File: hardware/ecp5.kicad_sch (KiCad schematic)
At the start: 6 parts, among them U3 ECP5U_12_CABGA256

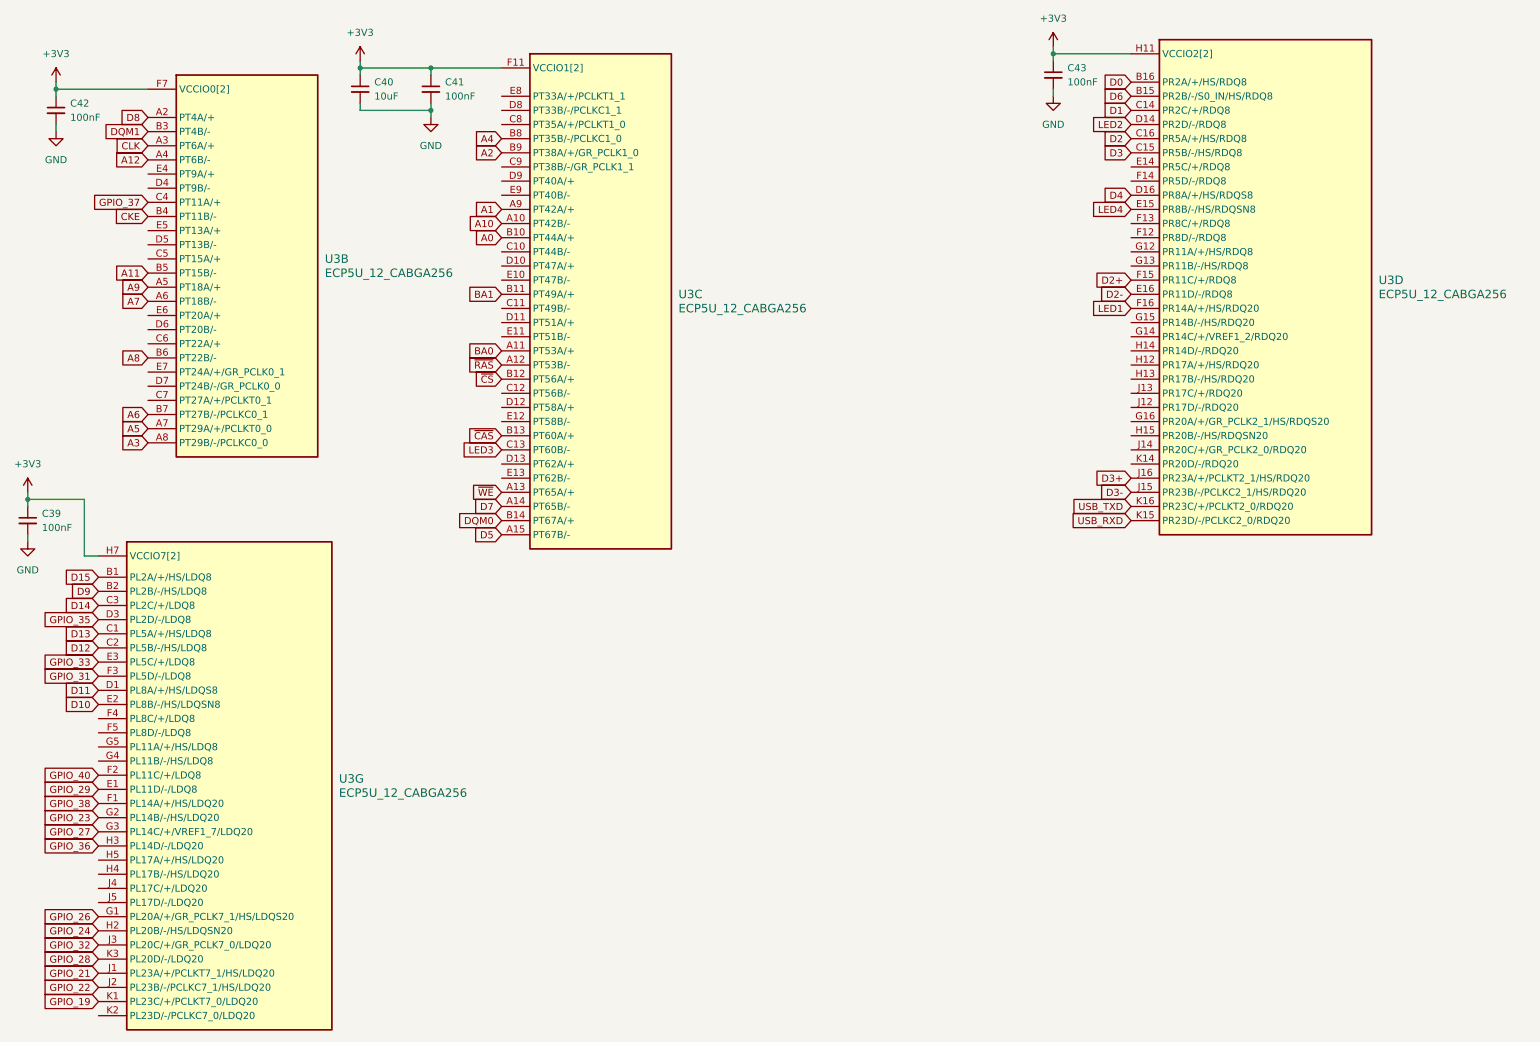
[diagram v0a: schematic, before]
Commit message: Pre-prod fixes
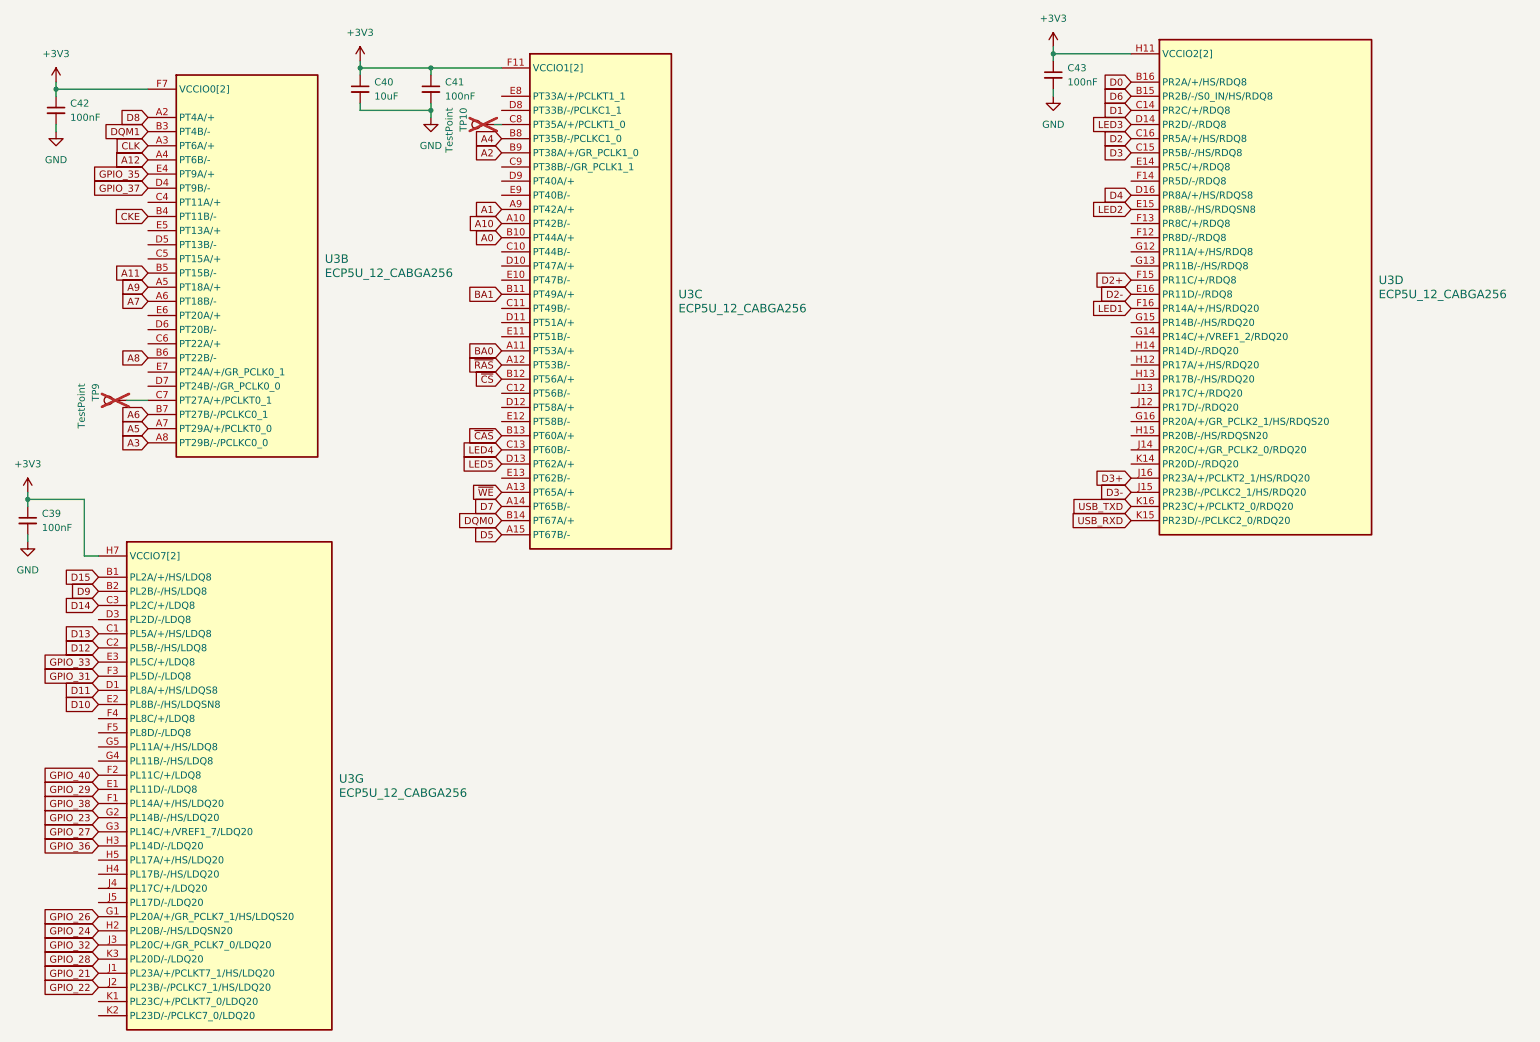
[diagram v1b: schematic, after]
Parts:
- added TP10, TP9: TestPoint, TestPoint:TestPoint_Pad_D2.0mm, symbol Connector:TestPoint
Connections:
- net GPIO_35: now also U3.E4 (PT9A/+); no longer U3.D3 (PL2D/-/LDQ8)
- net GPIO_37: now also U3.D4 (PT9B/-); no longer U3.C4 (PT11A/+)
- net LED2: now also U3.E15 (PR8B/-/HS/RDQSN8); no longer U3.D14 (PR2D/-/RDQ8)
- net LED3: now also U3.D14 (PR2D/-/RDQ8); no longer U3.C13 (PT60B/-)
- net LED4: now also U3.C13 (PT60B/-); no longer U3.E15 (PR8B/-/HS/RDQSN8)
- net at U3.C7 (PT27A/+/PCLKT0_1): now also TP9.1
- net at U3.C8 (PT35A/+/PCLKT1_0): now also TP10.1
- net LED5: now reaches U3.D13 (PT62A/+)
- net GPIO_19: no longer names the net of U3.K1 (PL23C/+/PCLKT7_0/LDQ20)
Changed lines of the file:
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@@
 	(wire
 		(pts
+			(xy 100.33 31.75) (xy 101.6 31.75)
+		)
+		(stroke
+			(width 0)
+			(type default)
+		)
+	)
+	(wire
+		(pts
 			(xy 21.59 31.75) (xy 21.59 33.02)
 		)
@@
 	(wire
 		(pts
+			(xy 34.29 81.28) (xy 38.1 81.28)
+		)
+		(stroke
+			(width 0)
+			(type default)
+		)
+	)
+	(wire
+		(pts
 			(xy 16.51 99.06) (xy 16.51 100.33)
 		)
@@
 		)
 	)
+	(global_label "GPIO_37"
+		(shape input)
+		(at 38.1 43.18 180)
+		(fields_autoplaced yes)
+		(effects
+			(font
+				(size 1.27 1.27)
+			)
+			(justify right)
+		)
+		(property "Intersheetrefs" "${INTERSHEET_REFS}"
+			(at 27.2529 43.18 0)
+			(effects
+				(font
+					(size 1.27 1.27)
+				)
+				(justify right)
+				(hide yes)
+			)
+		)
+	)
 	(global_label "GPIO_23"
 		(shape input)
@@
 		)
 	)
-	(global_label "GPIO_35"
-		(shape input)
-		(at 29.21 120.65 180)
-		(fields_autoplaced yes)
-		(effects
-			(font
-				(size 1.27 1.27)
-			)
-			(justify right)
-		)
-		(property "Intersheetrefs" "${INTERSHEET_REFS}"
-			(at 18.3629 120.65 0)
-			(effects
-				(font
-					(size 1.27 1.27)
-				)
-				(justify right)
-				(hide yes)
-			)
-		)
-	)
 	(global_label "D8"
 		(shape input)
@@
 		)
 	)
-	(global_label "GPIO_24"
+	(global_label "GPIO_35"
 		(shape input)
-		(at 29.21 176.53 180)
+		(at 38.1 40.64 180)
 		(fields_autoplaced yes)
 		(effects
@@
 		)
 		(property "Intersheetrefs" "${INTERSHEET_REFS}"
-			(at 18.3629 176.53 0)
+			(at 27.2529 40.64 0)
 			(effects
 				(font
@@
 		)
 	)
-	(global_label "D3"
+	(global_label "GPIO_24"
 		(shape input)
-		(at 214.63 36.83 180)
+		(at 29.21 176.53 180)
 		(fields_autoplaced yes)
 		(effects
@@
 		)
 		(property "Intersheetrefs" "${INTERSHEET_REFS}"
-			(at 209.1653 36.83 0)
+			(at 18.3629 176.53 0)
 			(effects
 				(font
@@
 		)
 	)
-	(global_label "GPIO_37"
+	(global_label "D3"
 		(shape input)
-		(at 38.1 45.72 180)
+		(at 214.63 36.83 180)
 		(fields_autoplaced yes)
 		(effects
@@
 		)
 		(property "Intersheetrefs" "${INTERSHEET_REFS}"
-			(at 27.2529 45.72 0)
+			(at 209.1653 36.83 0)
 			(effects
 				(font
@@
 		)
 	)
-	(global_label "LED2"
+	(global_label "LED3"
 		(shape input)
 		(at 214.63 31.75 180)
@@
 		)
 	)
-	(global_label "LED4"
+	(global_label "LED2"
 		(shape input)
 		(at 214.63 46.99 180)
@@
 		)
 	)
-	(global_label "GPIO_19"
+	(global_label "A0"
 		(shape input)
-		(at 29.21 189.23 180)
+		(at 101.6 52.07 180)
 		(fields_autoplaced yes)
 		(effects
@@
 		)
 		(property "Intersheetrefs" "${INTERSHEET_REFS}"
-			(at 18.3629 189.23 0)
+			(at 96.3167 52.07 0)
 			(effects
 				(font
@@
 		)
 	)
-	(global_label "A0"
+	(global_label "~{CS}"
 		(shape input)
-		(at 101.6 52.07 180)
+		(at 101.6 77.47 180)
 		(fields_autoplaced yes)
 		(effects
@@
 		)
 		(property "Intersheetrefs" "${INTERSHEET_REFS}"
-			(at 96.3167 52.07 0)
+			(at 96.1353 77.47 0)
 			(effects
 				(font
@@
 		)
 	)
-	(global_label "~{CS}"
+	(global_label "LED5"
 		(shape input)
-		(at 101.6 77.47 180)
+		(at 101.6 92.71 180)
 		(fields_autoplaced yes)
 		(effects
@@
 		)
 		(property "Intersheetrefs" "${INTERSHEET_REFS}"
-			(at 96.1353 77.47 0)
+			(at 93.9582 92.71 0)
 			(effects
 				(font
@@
 		)
 	)
-	(global_label "LED3"
+	(global_label "LED4"
 		(shape input)
 		(at 101.6 90.17 180)
@@
 	)
 	(symbol
+		(lib_id "Connector:TestPoint")
+		(at 34.29 81.28 90)
+		(unit 1)
+		(exclude_from_sim no)
+		(in_bom yes)
+		(on_board yes)
+		(dnp yes)
+		(property "Reference" "TP9"
+			(at 28.702 78.232 0)
+			(effects
+				(font
+					(size 1.27 1.27)
+				)
+				(justify right)
+			)
+		)
+		(property "Value" "TestPoint"
+			(at 26.162 78.232 0)
+			(effects
+				(font
+					(size 1.27 1.27)
+				)
+				(justify right)
+			)
+		)
+		(property "Footprint" "TestPoint:TestPoint_Pad_D2.0mm"
+			(at 34.29 76.2 0)
+			(effects
+				(font
+					(size 1.27 1.27)
+				)
+				(hide yes)
+			)
+		)
+		(property "Datasheet" "~"
+			(at 34.29 76.2 0)
+			(effects
+				(font
+					(size 1.27 1.27)
+				)
+				(hide yes)
+			)
+		)
+		(property "Description" "test point"
+			(at 34.29 81.28 0)
+			(effects
+				(font
+					(size 1.27 1.27)
+				)
+				(hide yes)
+			)
+		)
+		(pin "1"
+		)
+		(instances
+			(project "icepi-zero"
+				(path "/f88da08e-cf42-4d03-a08f-3f602fe6658d/17c9c9b3-f379-4e1f-a876-d3fcf0529a4d"
+					(reference "TP9")
+					(unit 1)
+				)
+			)
+		)
+	)
+	(symbol
 		(lib_id "josh:ECP5U_12_CABGA256")
 		(at 236.22 57.15 0)
@@
 					(unit 1)
 				)
+			)
+		)
+	)
+	(symbol
+		(lib_id "Connector:TestPoint")
+		(at 100.33 31.75 90)
+		(unit 1)
+		(exclude_from_sim no)
+		(in_bom yes)
+		(on_board yes)
+		(dnp yes)
+		(property "Reference" "TP10"
+			(at 94.742 28.702 0)
+			(effects
+				(font
+					(size 1.27 1.27)
+				)
+				(justify right)
+			)
+		)
+		(property "Value" "TestPoint"
+			(at 92.202 28.702 0)
+			(effects
+				(font
+					(size 1.27 1.27)
+				)
+				(justify right)
+			)
+		)
+		(property "Footprint" "TestPoint:TestPoint_Pad_D2.0mm"
+			(at 100.33 26.67 0)
+			(effects
+				(font
+					(size 1.27 1.27)
+				)
+				(hide yes)
+			)
+		)
+		(property "Datasheet" "~"
+			(at 100.33 26.67 0)
+			(effects
+				(font
+					(size 1.27 1.27)
+				)
+				(hide yes)
+			)
+		)
+		(property "Description" "test point"
+			(at 100.33 31.75 0)
+			(effects
+				(font
+					(size 1.27 1.27)
+				)
+				(hide yes)
+			)
+		)
+		(pin "1"
+		)
+		(instances
+			(project "icepi-zero"
+				(path "/f88da08e-cf42-4d03-a08f-3f602fe6658d/17c9c9b3-f379-4e1f-a876-d3fcf0529a4d"
+					(reference "TP10")
+					(unit 1)
+				)
